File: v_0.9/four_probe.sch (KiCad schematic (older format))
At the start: 79 parts, among them J1 Conn_01x30_Male, J2 RG, J3 CONSMA001-SMD-G, J4 CONSMA001-SMD-G, J5 CONSMA001-SMD-G, J6 CONSMA001-SMD-G, U1 LMC6482, U10 ADG704, U11 tmux1511, U2 AD623, U3 LMC6482, U4 AD623, U5 LMC6484, U6 LMC6484, U7 tmux1511, U8 ADG704, U9 ADG704

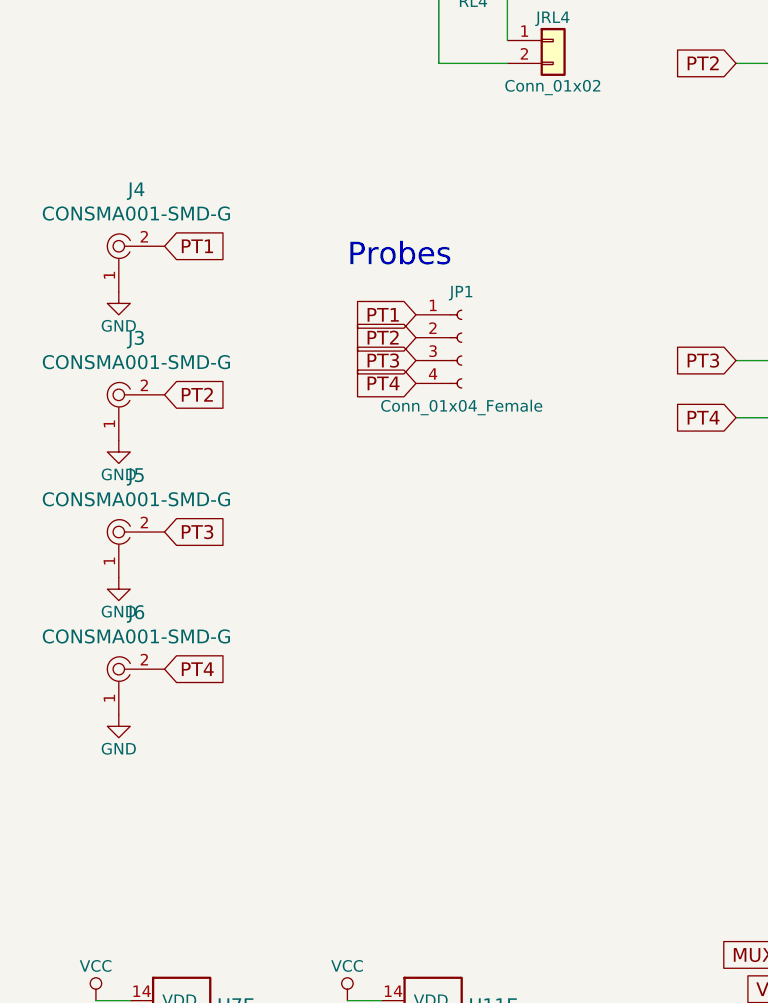
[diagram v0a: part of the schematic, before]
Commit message: update
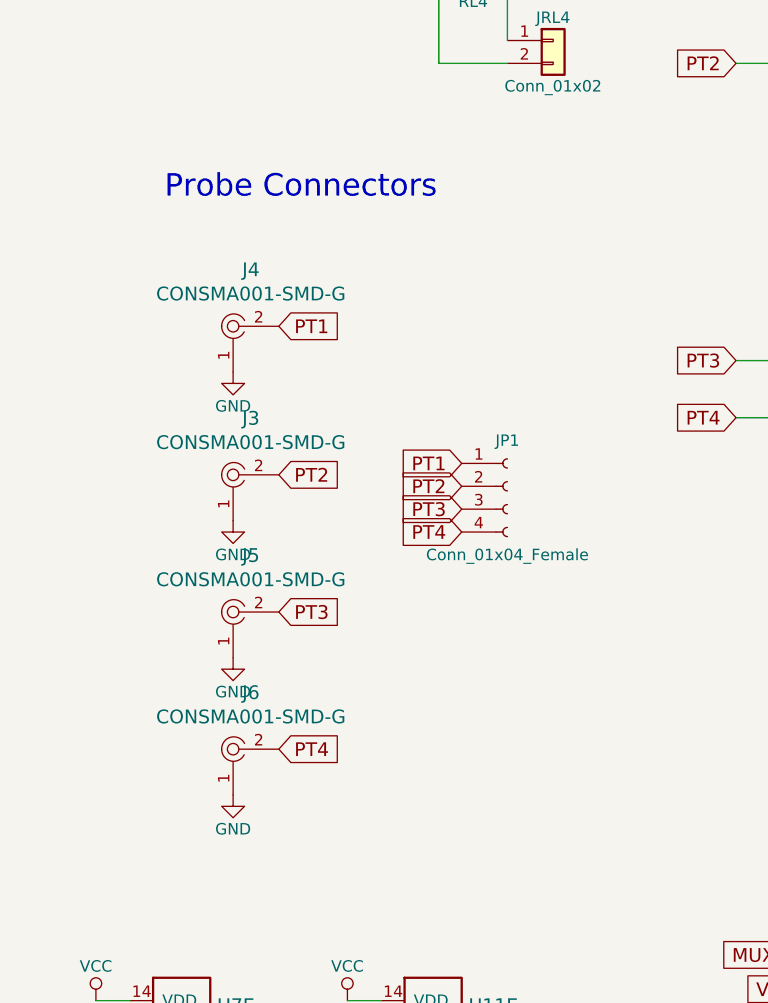
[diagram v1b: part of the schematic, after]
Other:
- note added: "Probe Connectors"
- note removed: "Probes"
- moved on the sheet: J3, J4, J5, J6, JP1

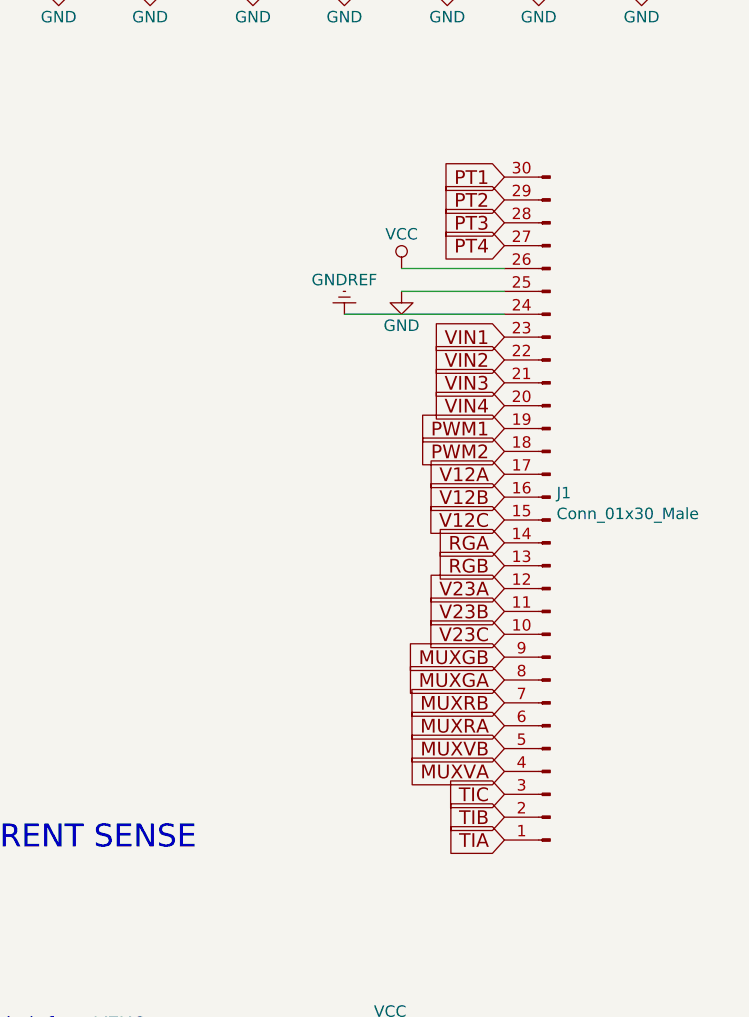
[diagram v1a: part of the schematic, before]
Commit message: update
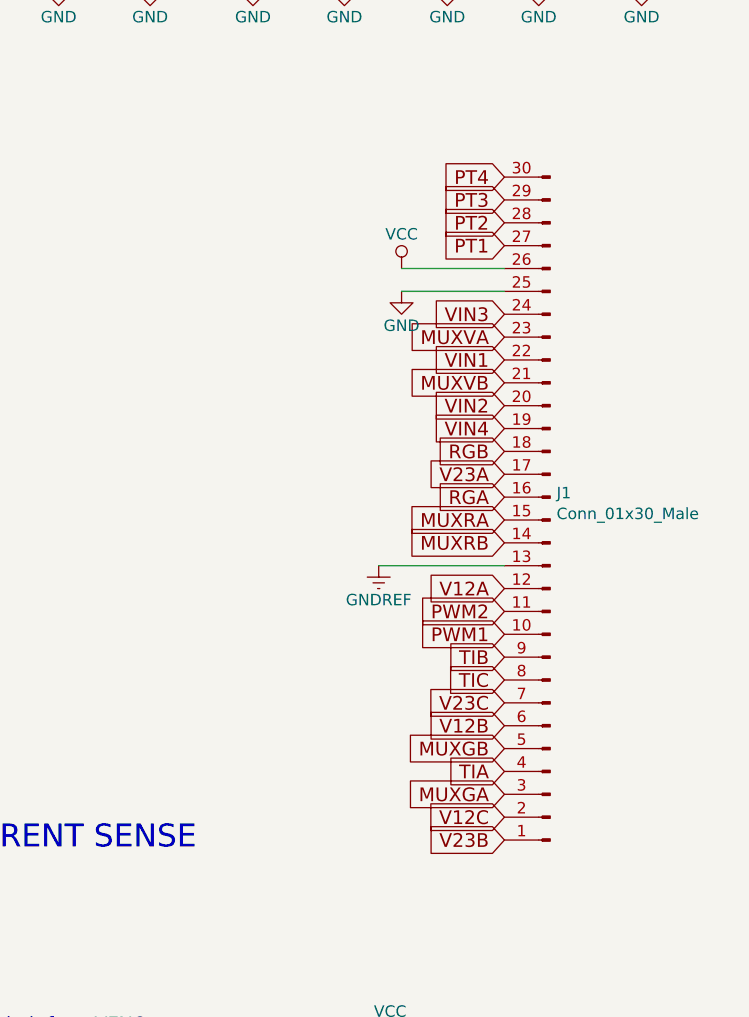
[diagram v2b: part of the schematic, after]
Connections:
- net GNDREF: now also J1.13 (Pin_13); no longer J1.24 (Pin_24)
- net MUXGA: now also J1.3 (Pin_3); no longer J1.8 (Pin_8)
- net MUXGB: now also J1.5 (Pin_5); no longer J1.9 (Pin_9)
- net MUXRA: now also J1.15 (Pin_15); no longer J1.6 (Pin_6)
- net MUXRB: now also J1.14 (Pin_14); no longer J1.7 (Pin_7)
- net MUXVA: now also J1.23 (Pin_23); no longer J1.4 (Pin_4)
- net MUXVB: now also J1.21 (Pin_21); no longer J1.5 (Pin_5)
- net P1: now also J1.27 (Pin_27); no longer J1.30 (Pin_30)
- net P2: now also J1.28 (Pin_28); no longer J1.29 (Pin_29)
- net P3: now also J1.29 (Pin_29); no longer J1.28 (Pin_28)
- net P4: now also J1.30 (Pin_30); no longer J1.27 (Pin_27)
- net PWM1: now also J1.10 (Pin_10); no longer J1.19 (Pin_19)
- net PWM2: now also J1.11 (Pin_11); no longer J1.18 (Pin_18)
- net RGA: now also J1.16 (Pin_16); no longer J1.14 (Pin_14)
- net RGB: now also J1.18 (Pin_18); no longer J1.13 (Pin_13)
- net TIA: now also J1.4 (Pin_4); no longer J1.1 (Pin_1)
- net TIB: now also J1.9 (Pin_9); no longer J1.2 (Pin_2)
- net TIC: now also J1.8 (Pin_8); no longer J1.3 (Pin_3)
- net V12A: now also J1.12 (Pin_12); no longer J1.17 (Pin_17)
- net V12B: now also J1.6 (Pin_6); no longer J1.16 (Pin_16)
- net V12C: now also J1.2 (Pin_2); no longer J1.15 (Pin_15)
- net V23A: now also J1.17 (Pin_17); no longer J1.12 (Pin_12)
- net V23B: now also J1.1 (Pin_1); no longer J1.11 (Pin_11)
- net V23C: now also J1.7 (Pin_7); no longer J1.10 (Pin_10)
- net VIN1: now also J1.22 (Pin_22); no longer J1.23 (Pin_23)
- net VIN2: now also J1.20 (Pin_20); no longer J1.22 (Pin_22)
- net VIN3: now also J1.24 (Pin_24); no longer J1.21 (Pin_21)
- net VIN4: now also J1.19 (Pin_19); no longer J1.20 (Pin_20)
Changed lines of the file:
@@
 	1    0    0    -1
 $EndComp
-Text GLabel 15500 3800 0    60   Input ~ 0
-V12C
 Text GLabel 15500 3600 0    60   Input ~ 0
-V12A
-Text GLabel 15500 3700 0    60   Input ~ 0
-V12B
+V23A
+Text GLabel 15500 5200 0    60   Input ~ 0
+V23B
+Text GLabel 15500 4600 0    60   Input ~ 0
+V23C
+Text GLabel 15500 4800 0    60   Input ~ 0
+MUXGB
+Text GLabel 15500 5000 0    60   Input ~ 0
+MUXGA
+Text GLabel 15500 3200 0    60   Input ~ 0
+MUXVB
 Text GLabel 15500 3000 0    60   Input ~ 0
-VIN1
-Text GLabel 15500 3100 0    60   Input ~ 0
-VIN2
-Text GLabel 15500 3200 0    60   Input ~ 0
-VIN3
-Text GLabel 15500 3300 0    60   Input ~ 0
-VIN4
-Text GLabel 15500 3400 0    60   Input ~ 0
-PWM1
-Text GLabel 15500 3500 0    60   Input ~ 0
-PWM2
-Text GLabel 15500 3900 0    60   Input ~ 0
-RGA
-Text GLabel 15500 4000 0    60   Input ~ 0
-RGB
-$Comp
-L four_probe-rescue:GNDREF-power #PWR0103
-U 1 1 5BD6F7F4
-P 14800 2900
-F 0 "#PWR0103" H 14800 2650 50  0001 C CNN
-F 1 "GNDREF" H 14800 2750 50  0000 C CNN
-F 2 "" H 14800 2900 50  0001 C CNN
-F 3 "" H 14800 2900 50  0001 C CNN
-	1    14800 2900
-	-1   0    0    1
-$EndComp
-Text GLabel 15500 4100 0    60   Input ~ 0
-V23A
-Text GLabel 15500 4200 0    60   Input ~ 0
-V23B
-Text GLabel 15500 4300 0    60   Input ~ 0
-V23C
-Text GLabel 15500 4400 0    60   Input ~ 0
-MUXGB
+MUXVA
+Text GLabel 15500 4900 0    60   Input ~ 0
+TIA
 Text GLabel 15500 4500 0    60   Input ~ 0
-MUXGA
-Text GLabel 15500 4600 0    60   Input ~ 0
-MUXRB
-Text GLabel 15500 4700 0    60   Input ~ 0
-MUXRA
-Text GLabel 15500 4800 0    60   Input ~ 0
-MUXVB
-Text GLabel 15500 4900 0    60   Input ~ 0
-MUXVA
-Text GLabel 15500 5100 0    60   Input ~ 0
-TIB
-Text GLabel 15500 5200 0    60   Input ~ 0
-TIA
-Text GLabel 15500 5000 0    60   Input ~ 0
 TIC
 $Comp
@@
 	-1   0    0    1
 $EndComp
+Text GLabel 15500 2600 0    60   Input ~ 0
+PT1
+Text GLabel 15500 2500 0    60   Input ~ 0
+PT2
+Text GLabel 15500 2400 0    60   Input ~ 0
+PT3
 Text GLabel 15500 2300 0    60   Input ~ 0
-PT1
-Text GLabel 15500 2400 0    60   Input ~ 0
-PT2
-Text GLabel 15500 2500 0    60   Input ~ 0
-PT3
-Text GLabel 15500 2600 0    60   Input ~ 0
 PT4
 Wire Wire Line
@@
 	15050 2800 15500 2800
 Wire Wire Line
-	14800 2900 15500 2900
+	15500 4000 14950 4000
+Text GLabel 15500 3400 0    60   Input ~ 0
+VIN4
+Text GLabel 15500 2900 0    60   Input ~ 0
+VIN3
+Text GLabel 15500 3300 0    60   Input ~ 0
+VIN2
+Text GLabel 15500 3100 0    60   Input ~ 0
+VIN1
+Text GLabel 15500 3800 0    60   Input ~ 0
+MUXRA
+Text GLabel 15500 3900 0    60   Input ~ 0
+MUXRB
+$Comp
+L four_probe-rescue:GNDREF-power #PWR0103
+U 1 1 5BD6F7F4
+P 14950 4000
+F 0 "#PWR0103" H 14950 3750 50  0001 C CNN
+F 1 "GNDREF" H 14950 3850 50  0000 C CNN
+F 2 "" H 14950 4000 50  0001 C CNN
+F 3 "" H 14950 4000 50  0001 C CNN
+	1    14950 4000
+	1    0    0    -1
+$EndComp
+Text GLabel 15500 3500 0    60   Input ~ 0
+RGB
+Text GLabel 15500 3700 0    60   Input ~ 0
+RGA
+Text GLabel 15500 4200 0    60   Input ~ 0
+PWM2
+Text GLabel 15500 4300 0    60   Input ~ 0
+PWM1
+Text GLabel 15500 4700 0    60   Input ~ 0
+V12B
+Text GLabel 15500 4100 0    60   Input ~ 0
+V12A
+Text GLabel 15500 5100 0    60   Input ~ 0
+V12C
+Text GLabel 15500 4400 0    60   Input ~ 0
+TIB
 $EndSCHEMATC
